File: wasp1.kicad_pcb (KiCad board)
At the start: 2 copper layers, 162.6 x 175.3 mm, 46 parts

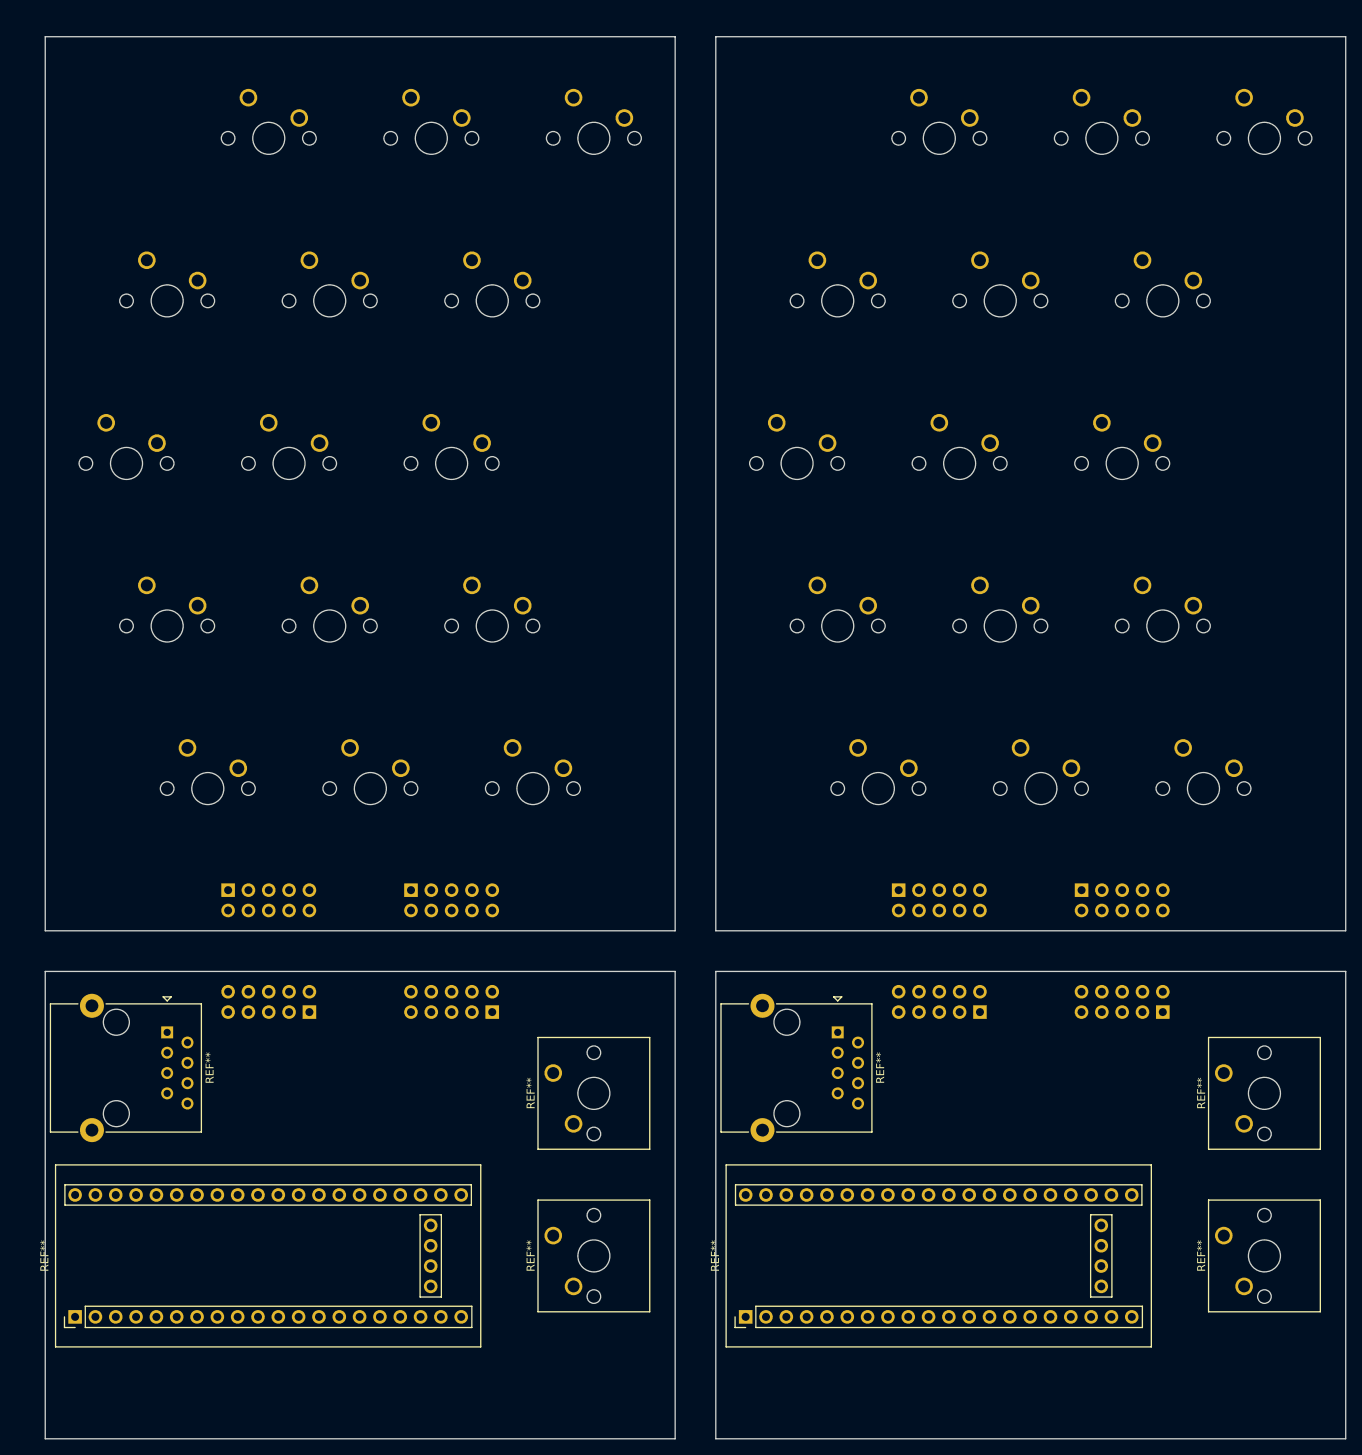
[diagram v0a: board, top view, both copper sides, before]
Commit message: Cutouts
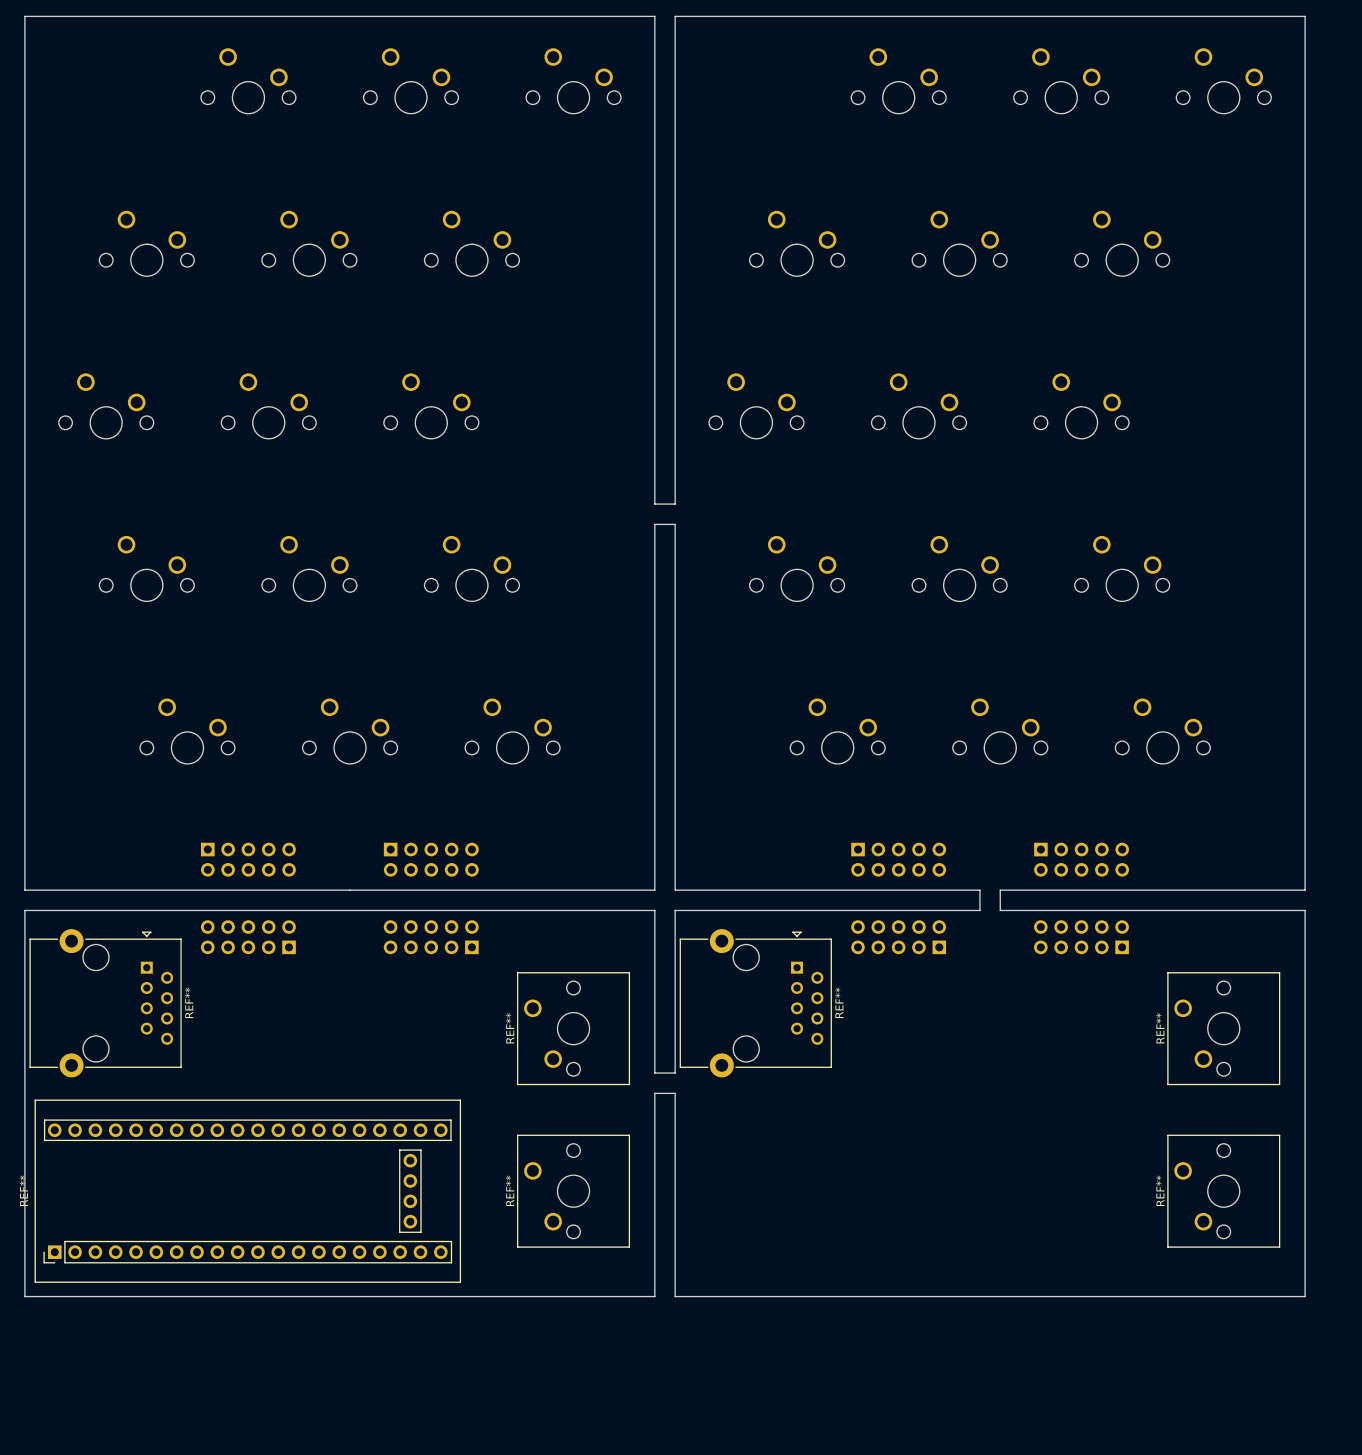
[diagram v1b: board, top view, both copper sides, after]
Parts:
- removed the REF** at (102.8, 175.3)
- moved REF** 9.56 mm to (127.0, 129.1)
- moved REF** 9.56 mm to (149.8, 129.1)
- moved REF** 9.56 mm to (157.5, 157.0)
- moved REF** 9.56 mm to (157.5, 136.7)
- moved REF** 9.56 mm to (109.2, 131.6)
- moved REF** 8.48 mm to (16.4, 167.2)
- moved REF** 8.48 mm to (76.2, 136.7)
- moved REF** 8.48 mm to (68.6, 129.1)
- moved REF** 8.48 mm to (76.2, 157.0)
- moved REF** 8.48 mm to (45.7, 129.1)
- moved REF** 8.48 mm to (27.9, 131.6)
- moved REF** 7.18 mm to (147.3, 38.1)
- moved REF** 7.18 mm to (139.7, 17.8)
- moved REF** 7.18 mm to (147.3, 78.7)
- moved REF** 7.18 mm to (127.0, 38.1)
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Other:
- board size 162.6 x 175.3 mm -> 160 x 160 mm

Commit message: All components
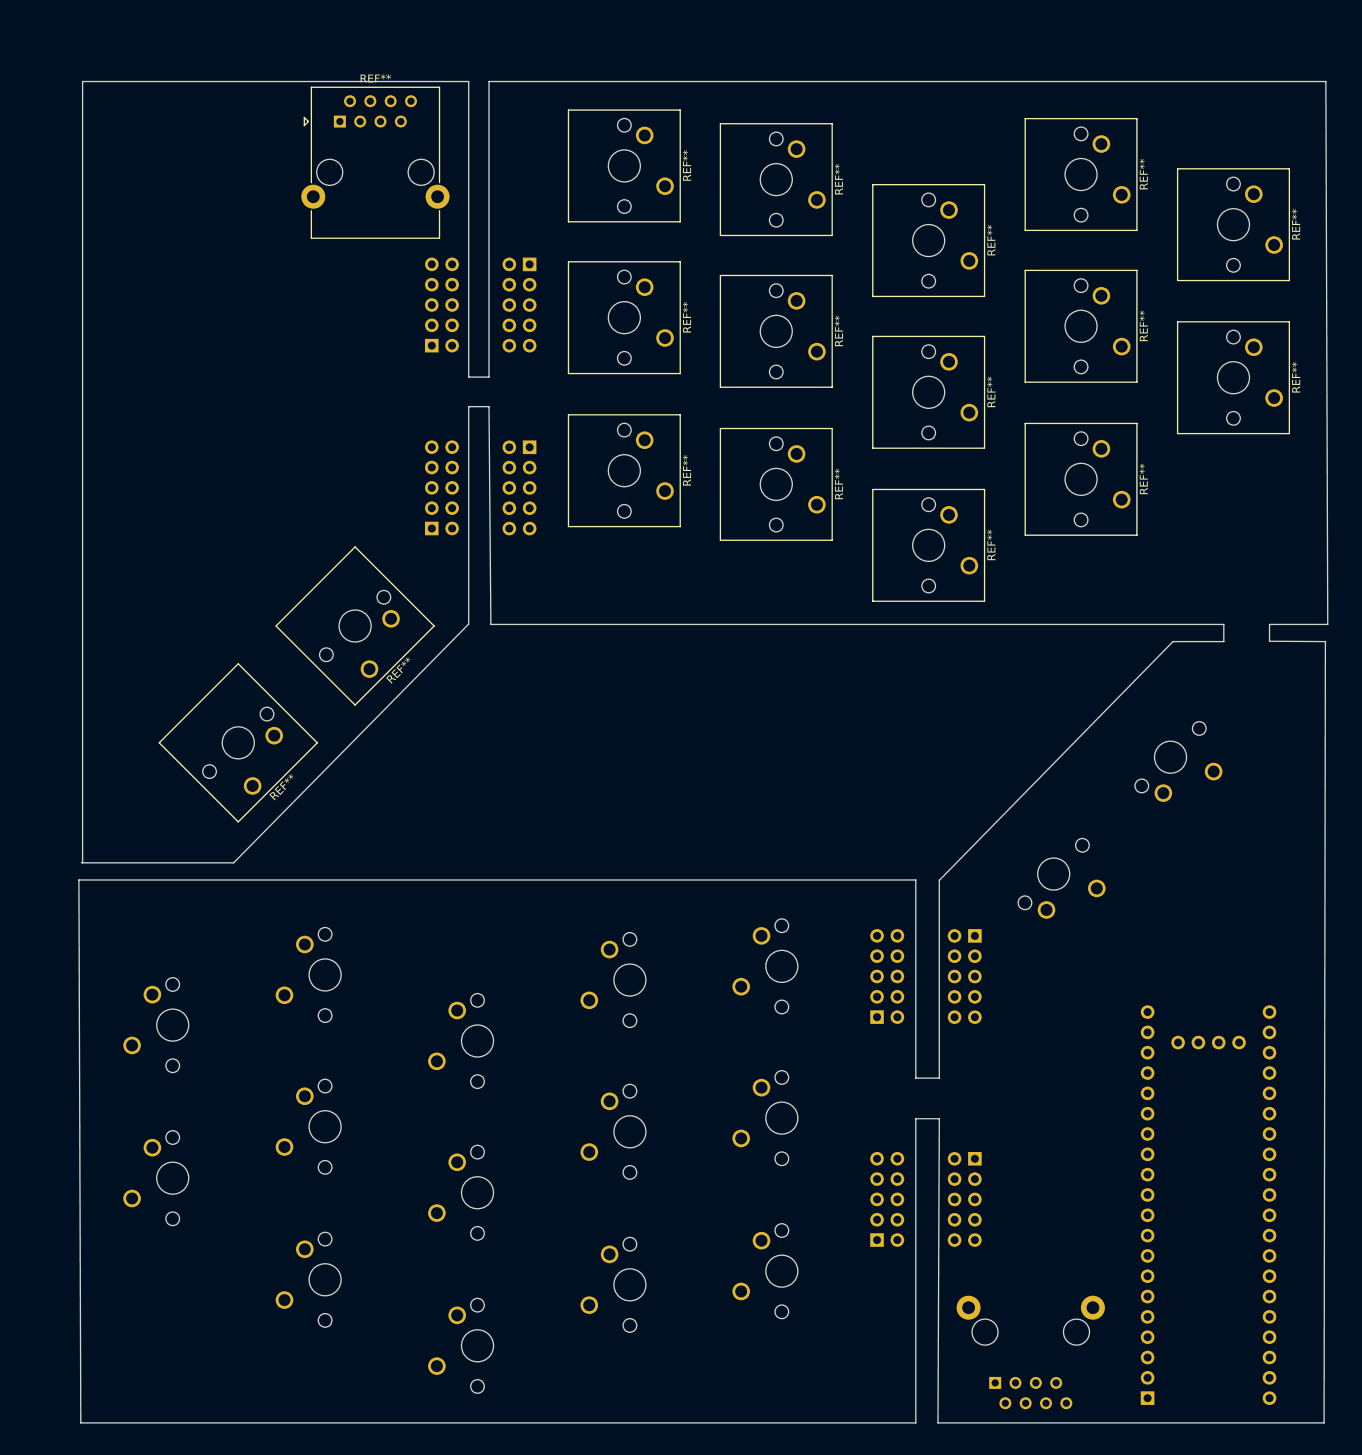
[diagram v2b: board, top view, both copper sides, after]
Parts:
- removed the REF** at (111.8, 99.1)
- removed the REF** at (142.2, 58.4)
- removed the REF** at (160.0, 17.8)
- removed the REF** at (119.4, 17.8)
- removed the REF** at (116.8, 116.8)
- removed the REF** at (40.6, 58.4)
- removed the REF** at (132.1, 99.1)
- removed the REF** at (38.1, 17.8)
- removed the REF** at (106.7, 78.7)
- removed the REF** at (45.7, 38.1)
- removed the REF** at (61.0, 58.4)
- removed the REF** at (20.3, 58.4)
- removed the REF** at (127.0, 129.1)
- removed the REF** at (147.3, 38.1)
- removed the REF** at (139.7, 17.8)
- removed the REF** at (106.7, 38.1)
- removed the REF** at (25.4, 38.1)
- removed the REF** at (149.8, 129.1)
- removed the REF** at (147.3, 78.7)
- removed the REF** at (58.4, 17.8)
- removed the REF** at (127.0, 38.1)
- removed the REF** at (66.0, 78.7)
- removed the REF** at (121.9, 58.4)
- removed the REF** at (78.7, 17.8)
- removed the REF** at (76.2, 157.0)
- removed the REF** at (101.6, 58.4)
- removed the REF** at (25.4, 78.7)
- removed the REF** at (139.7, 116.8)
- removed the REF** at (152.4, 99.1)
- removed the REF** at (127.0, 78.7)
- removed the REF** at (157.5, 157.0)
- removed the REF** at (157.5, 136.7)
- removed the REF** at (66.0, 38.1)
- removed the REF** at (45.7, 78.7)
- added REF**: SW_Cherry_MX_1.00u_PCB, Button_Switch_Keyboard:SW_Cherry_MX_1.00u_PCB, F.Cu at (149.8, 73.1)
- added REF**: SW_Cherry_MX_1.00u_PCB, Button_Switch_Keyboard:SW_Cherry_MX_1.00u_PCB, F.Cu at (168.8, 60.4)
- added REF**: SW_Cherry_MX_1.00u_PCB, Button_Switch_Keyboard:SW_Cherry_MX_1.00u_PCB, F.Cu at (41.2, 108.9)
- added REF**: SW_Cherry_MX_1.00u_PCB, Button_Switch_Keyboard:SW_Cherry_MX_1.00u_PCB, F.Cu at (130.8, 62.2)
- added REF**: SW_Cherry_MX_1.00u_PCB, Button_Switch_Keyboard:SW_Cherry_MX_1.00u_PCB, F.Cu at (149.8, 54.0)
- added REF**: SW_Cherry_MX_1.00u_PCB, Button_Switch_Keyboard:SW_Cherry_MX_1.00u_PCB, F.Cu at (130.8, 43.3)
- added REF**: SW_Cherry_MX_1.00u_PCB, Button_Switch_Keyboard:SW_Cherry_MX_1.00u_PCB, F.Cu at (55.8, 94.3)
- added REF**: SW_Cherry_MX_1.00u_PCB, Button_Switch_Keyboard:SW_Cherry_MX_1.00u_PCB, F.Cu at (111.7, 54.6)
- added REF**: SW_Cherry_MX_1.00u_PCB, Button_Switch_Keyboard:SW_Cherry_MX_1.00u_PCB, B.Cu at (64.2, 143.3)
- added REF**: SW_Cherry_MX_1.00u_PCB, Button_Switch_Keyboard:SW_Cherry_MX_1.00u_PCB, F.Cu at (92.7, 33.9)
- added REF**: SW_Cherry_MX_1.00u_PCB, Button_Switch_Keyboard:SW_Cherry_MX_1.00u_PCB, B.Cu at (64.2, 181.4)
- added REF**: SW_Cherry_MX_1.00u_PCB, Button_Switch_Keyboard:SW_Cherry_MX_1.00u_PCB, B.Cu at (26.1, 160.5)
- added REF**: SW_Cherry_MX_1.00u_PCB, Button_Switch_Keyboard:SW_Cherry_MX_1.00u_PCB, B.Cu at (64.2, 162.3)
- added REF**: SW_Cherry_MX_1.00u_PCB, Button_Switch_Keyboard:SW_Cherry_MX_1.00u_PCB, B.Cu at (45.1, 135.1)
- added REF**: SW_Cherry_MX_1.00u_PCB, Button_Switch_Keyboard:SW_Cherry_MX_1.00u_PCB, B.Cu at (45.1, 154.0)
- added REF**: SW_Cherry_MX_1.00u_PCB, Button_Switch_Keyboard:SW_Cherry_MX_1.00u_PCB, B.Cu at (83.2, 173.8)
- added REF**: PinHeader_2x05_P2.54mm_Horizontal, Connector_PinHeader_2.54mm:PinHeader_2x05_P2.54mm_Horizontal, B.Cu at (75.8, 43.7)
- added REF**: SW_Cherry_MX_1.00u_PCB, Button_Switch_Keyboard:SW_Cherry_MX_1.00u_PCB, F.Cu at (92.7, 72.0)
- added REF**: SW_Cherry_MX_1.00u_PCB, Button_Switch_Keyboard:SW_Cherry_MX_1.00u_PCB, B.Cu at (26.1, 141.3)
- added REF**: SW_Cherry_MX_1.00u_PCB, Button_Switch_Keyboard:SW_Cherry_MX_1.00u_PCB, B.Cu at (45.1, 173.2)
- added REF**: SW_Cherry_MX_1.00u_PCB, Button_Switch_Keyboard:SW_Cherry_MX_1.00u_PCB, B.Cu at (83.2, 135.7)
- added REF**: PinHeader_2x05_P2.54mm_Horizontal, Connector_PinHeader_2.54mm:PinHeader_2x05_P2.54mm_Horizontal, B.Cu at (75.8, 66.6)
- added REF**: SW_Cherry_MX_1.00u_PCB, Button_Switch_Keyboard:SW_Cherry_MX_1.00u_PCB, B.Cu at (83.2, 154.7)
- added REF**: SW_Cherry_MX_1.00u_PCB, Button_Switch_Keyboard:SW_Cherry_MX_1.00u_PCB, F.Cu at (168.8, 41.3)
- added REF**: SW_Cherry_MX_1.00u_PCB, Button_Switch_Keyboard:SW_Cherry_MX_1.00u_PCB, B.Cu at (161.3, 107.1)
- added REF**: PinHeader_2x05_P2.54mm_Horizontal, Connector_PinHeader_2.54mm:PinHeader_2x05_P2.54mm_Horizontal, B.Cu at (63.6, 53.9)
- added REF**: PinHeader_2x05_P2.54mm_Horizontal, Connector_PinHeader_2.54mm:PinHeader_2x05_P2.54mm_Horizontal, B.Cu at (63.6, 76.7)
- added REF**: SW_Cherry_MX_1.00u_PCB, Button_Switch_Keyboard:SW_Cherry_MX_1.00u_PCB, F.Cu at (111.7, 73.7)
- added REF**: SW_Cherry_MX_1.00u_PCB, Button_Switch_Keyboard:SW_Cherry_MX_1.00u_PCB, F.Cu at (149.8, 35.0)
- added REF**: SW_Cherry_MX_1.00u_PCB, Button_Switch_Keyboard:SW_Cherry_MX_1.00u_PCB, F.Cu at (130.8, 81.4)
- added REF**: SW_Cherry_MX_1.00u_PCB, Button_Switch_Keyboard:SW_Cherry_MX_1.00u_PCB, F.Cu at (92.7, 52.9)
- added REF**: SW_Cherry_MX_1.00u_PCB, Button_Switch_Keyboard:SW_Cherry_MX_1.00u_PCB, F.Cu at (111.7, 35.6)
- REF** (x3): moved to B.Cu
- moved REF** 137.8 mm to (153.0, 185.4), turned to 0 degrees
- moved REF** 120.2 mm to (52.1, 25.8), turned to 0 degrees
- moved REF** 118.1 mm to (134.0, 183.5), turned to 0 degrees
- moved REF** 102.4 mm to (102.2, 172.1), turned to -90 degrees
- moved REF** 96.9 mm to (119.2, 165.7), turned to 0 degrees
- moved REF** 89.7 mm to (131.4, 155.5), turned to 180 degrees
- moved REF** 74.5 mm to (102.2, 153.0), turned to -90 degrees
- moved REF** 72.1 mm to (146.7, 121.7), turned to 45 degrees
- moved REF** 64.3 mm to (119.2, 137.8), turned to 0 degrees
- moved REF** 62.9 mm to (131.4, 127.6), turned to 180 degrees
- moved REF** 46.8 mm to (102.2, 134.0), turned to -90 degrees
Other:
- board size 160 x 160 mm -> 156.1 x 167.7 mm
- board text added: "PinHeader_2x05_P2.54mm_Horizontal"
